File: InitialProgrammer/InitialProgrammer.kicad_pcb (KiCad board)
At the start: 2 copper layers, 24 x 20 mm, 7 parts, among them CN1 YZ29115060P-02, CN2 YZ29115060P-02, CN3 YZ29115060P-02, CN4 YZ29115060P-02, CN5 YZ29115060P-02, CN6 YZ29115060P-02

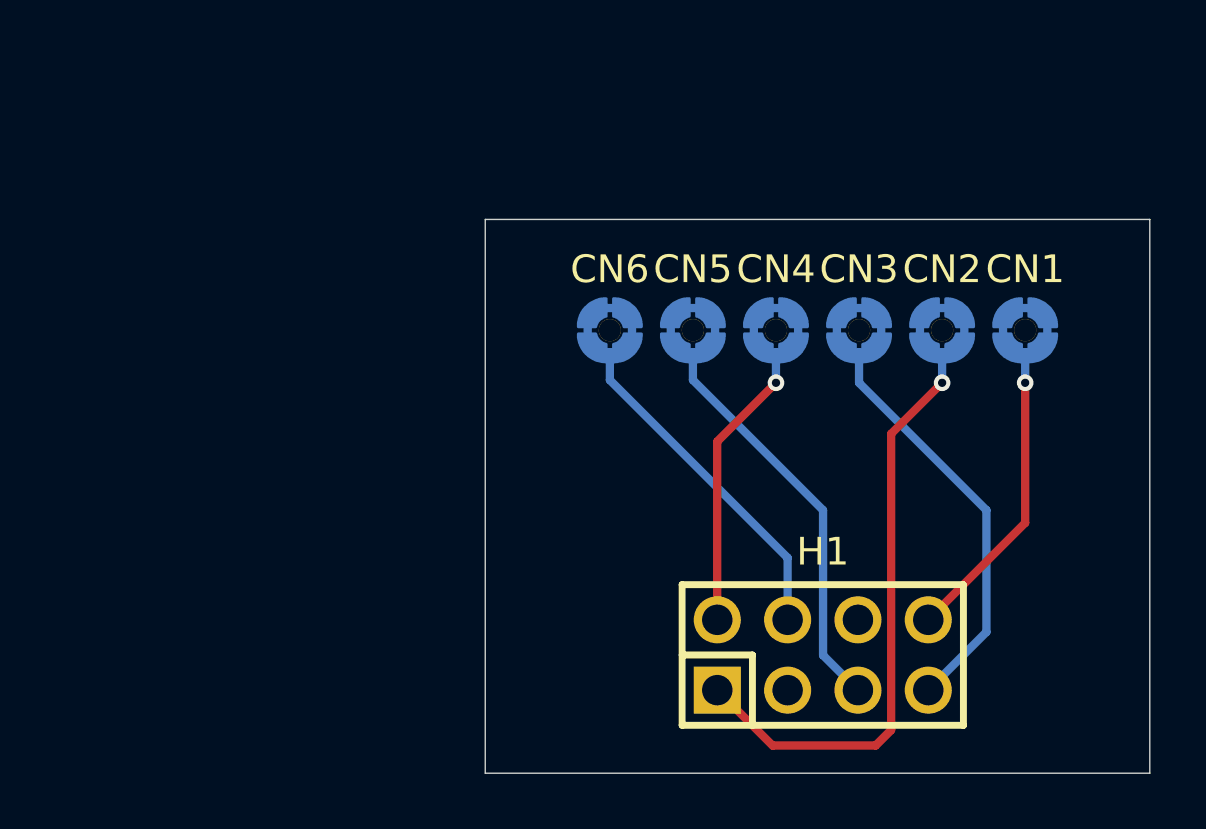
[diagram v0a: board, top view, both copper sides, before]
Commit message: update
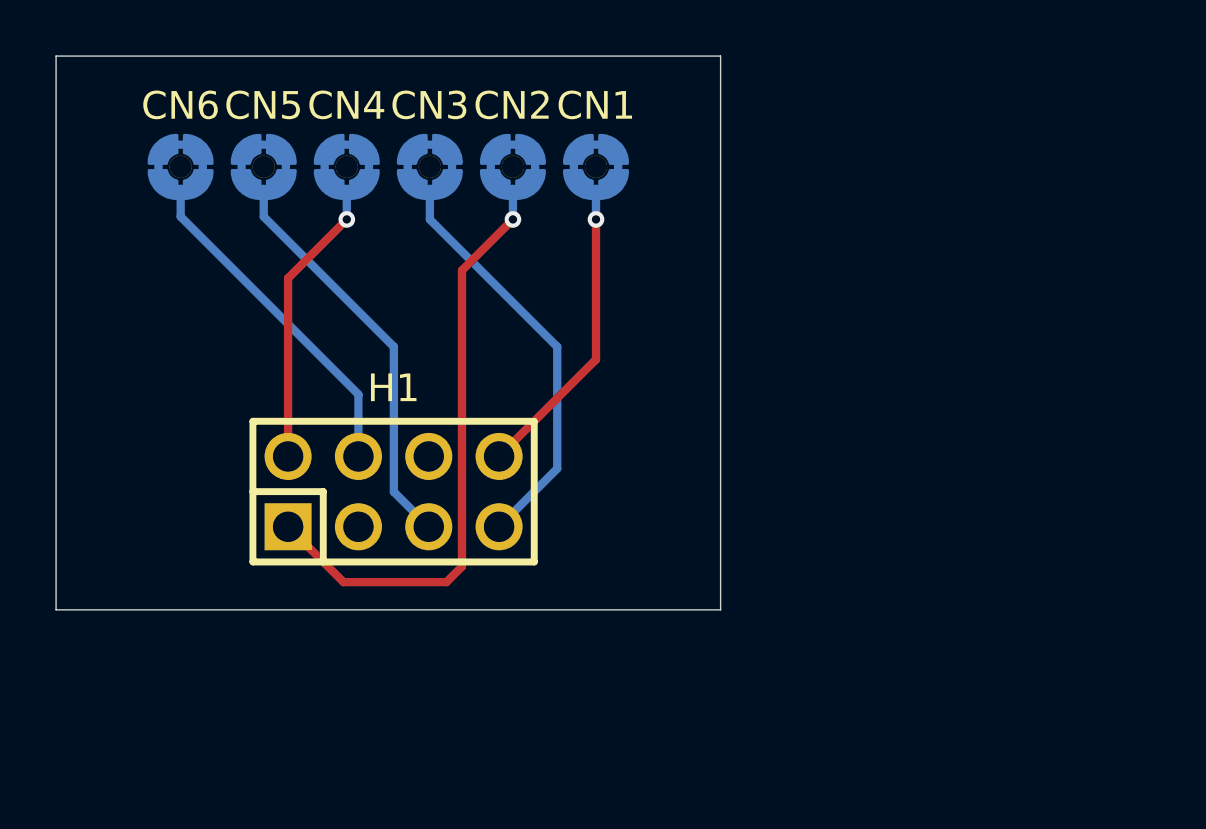
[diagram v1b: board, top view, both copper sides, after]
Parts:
- moved CN1 16.6 mm to (152.0, 88.1)
- moved CN2 16.6 mm to (149.0, 88.1)
- moved CN3 16.6 mm to (146.0, 88.1)
- moved CN4 16.6 mm to (143.0, 88.1)
- moved CN5 16.6 mm to (140.0, 88.1)
- moved CN6 16.6 mm to (137.0, 88.1)
- moved H1 16.6 mm to (144.7, 99.8)
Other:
- board text added: "Converts https://www.tindie.com/products/snakeye/usb-programmer-for-esp8266esp32/ to pad format used by board."
